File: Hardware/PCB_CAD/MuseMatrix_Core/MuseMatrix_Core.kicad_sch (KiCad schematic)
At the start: 0 parts

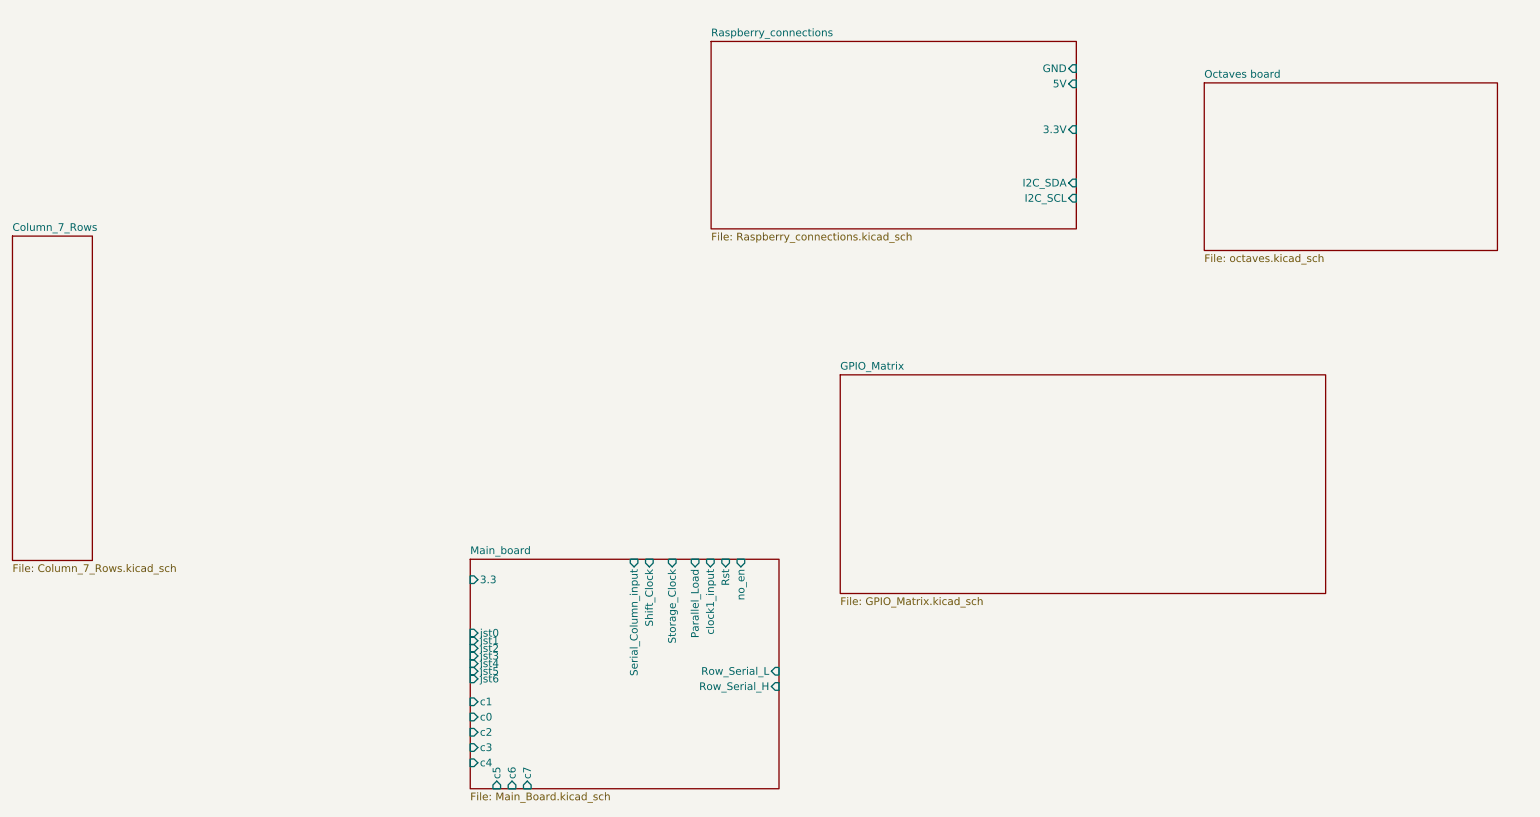
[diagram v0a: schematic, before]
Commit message: more pcb edit
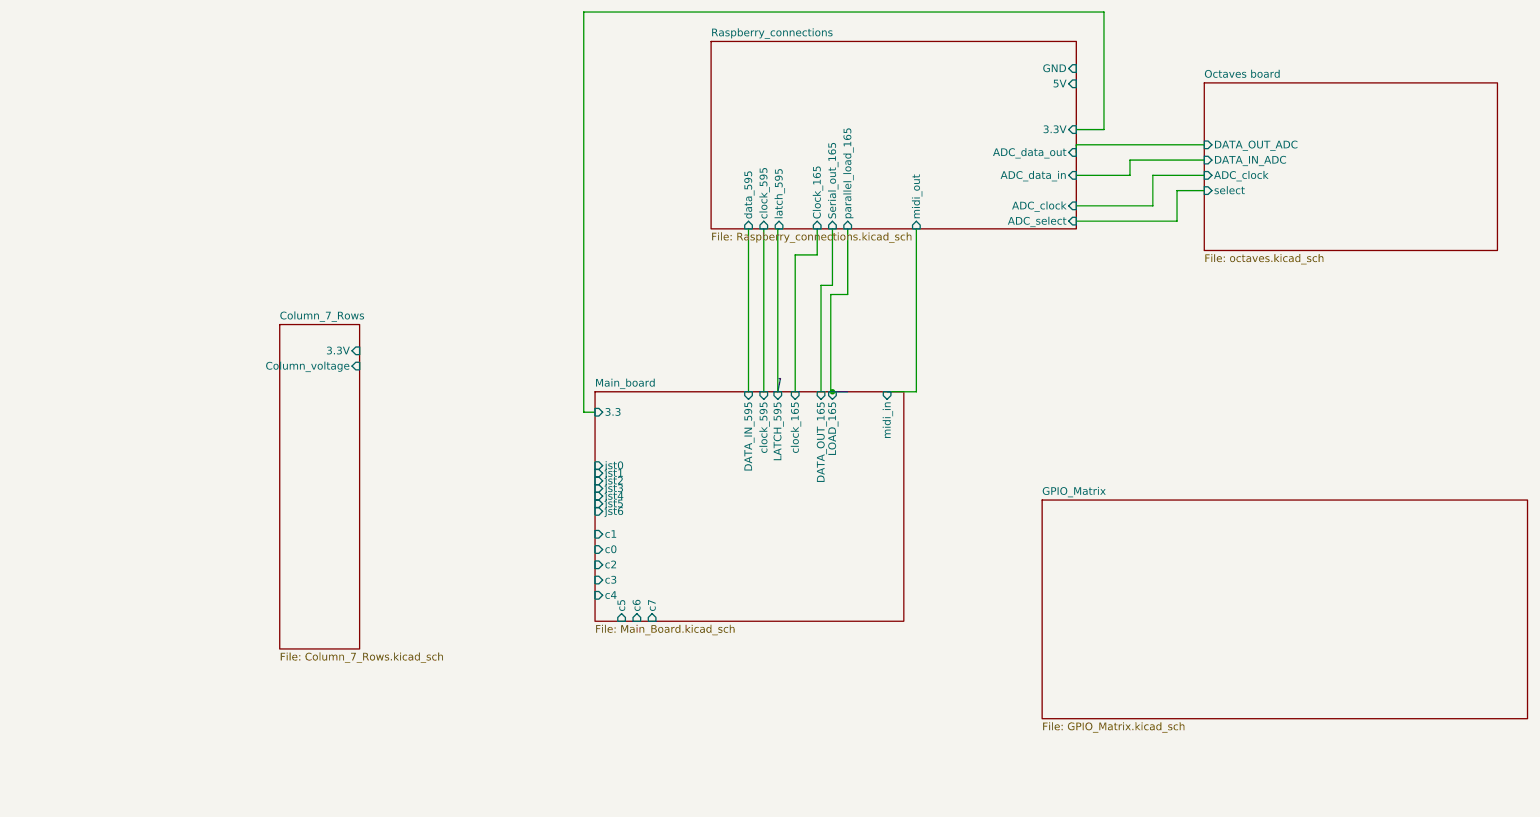
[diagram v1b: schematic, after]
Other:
- sheet Column_7_Rows ports: added 3.3V, Column_voltage; removed none
- sheet Main_board ports: added DATA_IN_595, DATA_OUT_165, LATCH_595, LOAD_165, clock_165, clock_595, midi_in; removed Parallel_Load, Row_Serial_H, Row_Serial_L, Rst, Serial_Column_input, Shift_Clock, Storage_Clock, clock1_input, no_en
- sheet Octaves board ports: added ADC_clock, DATA_IN_ADC, DATA_OUT_ADC, select; removed none
- sheet Raspberry_connections ports: added ADC_clock, ADC_data_in, ADC_data_out, ADC_select, Clock_165, Serial_out_165, clock_595, data_595, latch_595, midi_out, parallel_load_165; removed I2C_SCL, I2C_SDA
